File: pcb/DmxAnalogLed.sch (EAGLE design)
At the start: 53 parts, among them IC2 7805TV, J1 RS485, J2 POWER_JACKPTH, J3 RS485, Q1 16MHz 10ppm, U1 ARDUINO_LEONARDO-REV3B_SMARTP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, U2 SN75176ASOIC, X1 USBPTH

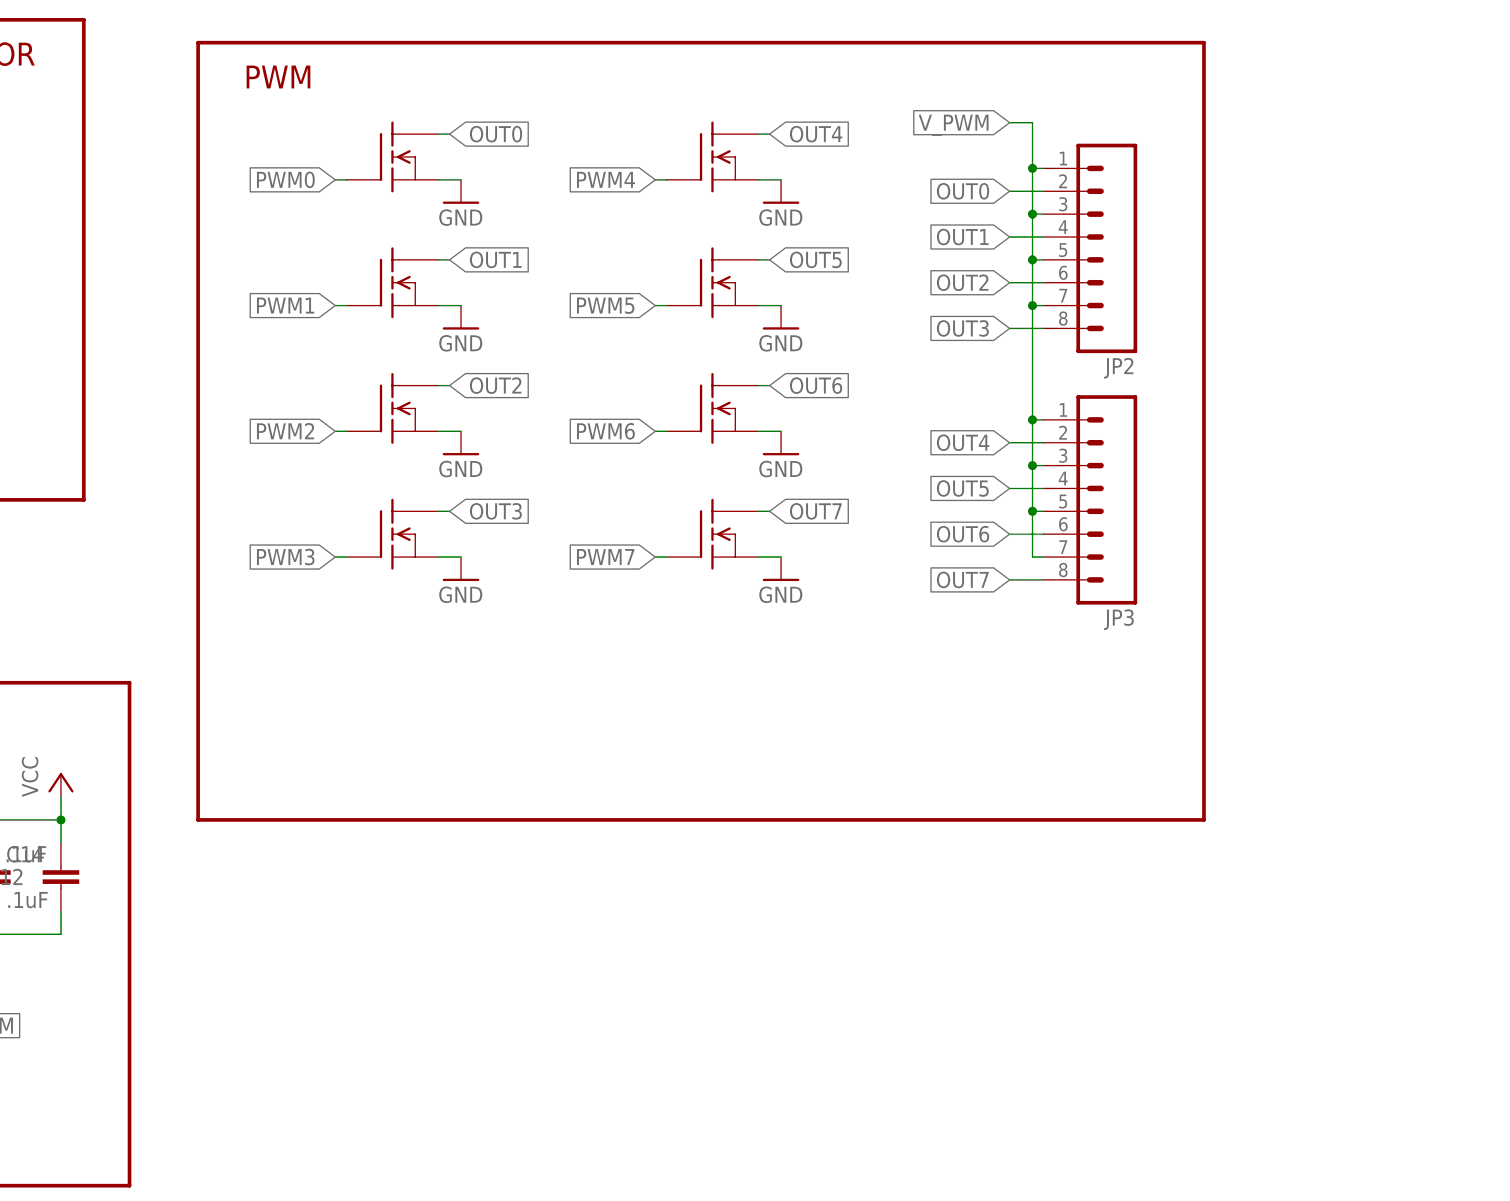
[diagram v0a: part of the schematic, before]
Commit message: Almost ready for a re-release of RevA
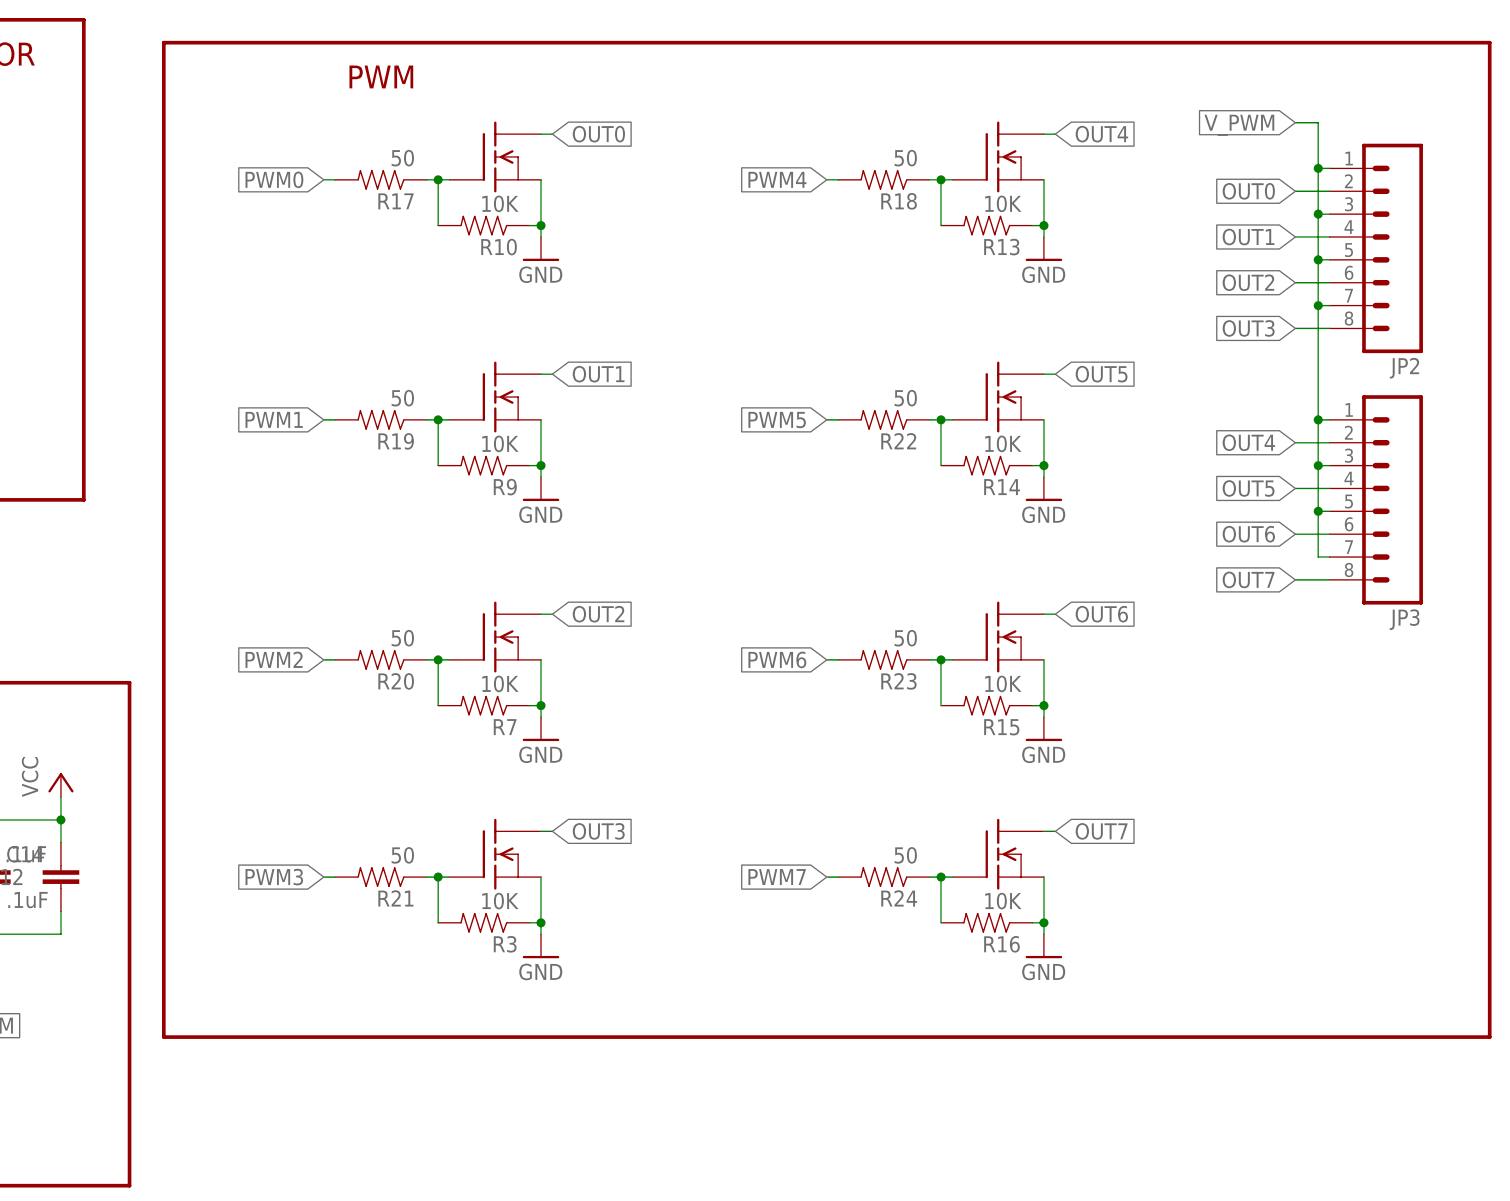
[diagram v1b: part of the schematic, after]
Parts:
- added R10, R13, R14, R15, R16, R3, R7, R9: 10K, SparkFun:RESISTOR
- added R17, R18, R19, R20, R21, R22, R23, R24: 50, SparkFun:RESISTOR
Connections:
- new net PWM0_MID: R10.2, R17.1, U$1.G
- new net PWM1_MID: R19.1, R9.2, U$3.G
- new net PWM2_MID: R20.1, R7.2, U$4.G
- new net PWM3_MID: R21.1, R3.2, U$5.G
- new net PWM4_MID: R13.2, R18.1, U$6.G
- new net PWM5_MID: R14.2, R22.1, U$7.G
- new net PWM6_MID: R15.2, R23.1, U$8.G
- new net PWM7_MID: R16.2, R24.1, U$9.G
- net GND: now also R10.1, R13.1, R14.1, R15.1, R16.1, R3.1, R7.1, R9.1
- net PWM0: now also R17.2; no longer U$1.G
- net PWM1: now also R19.2; no longer U$3.G
- net PWM2: now also R20.2; no longer U$4.G
- net PWM3: now also R21.2; no longer U$5.G
- net PWM4: now also R18.2; no longer U$6.G
- net PWM5: now also R22.2; no longer U$7.G
- net PWM6: now also R23.2; no longer U$8.G
- net PWM7: now also R24.2; no longer U$9.G
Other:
- moved on the sheet: JP2, JP3
